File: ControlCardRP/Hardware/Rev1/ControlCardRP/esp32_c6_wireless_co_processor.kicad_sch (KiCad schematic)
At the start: 22 parts, among them J6 ESP_PROG_UART, J7 ESP_PROG_JTAG, J8 ESP_IO, SW103 NRST, SW104 NRST, U5 ESP32-C6-MINI-1

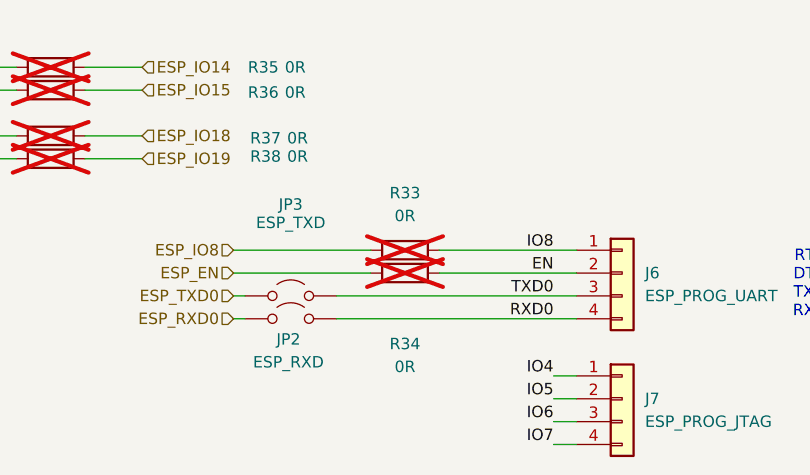
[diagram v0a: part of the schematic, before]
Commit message: A
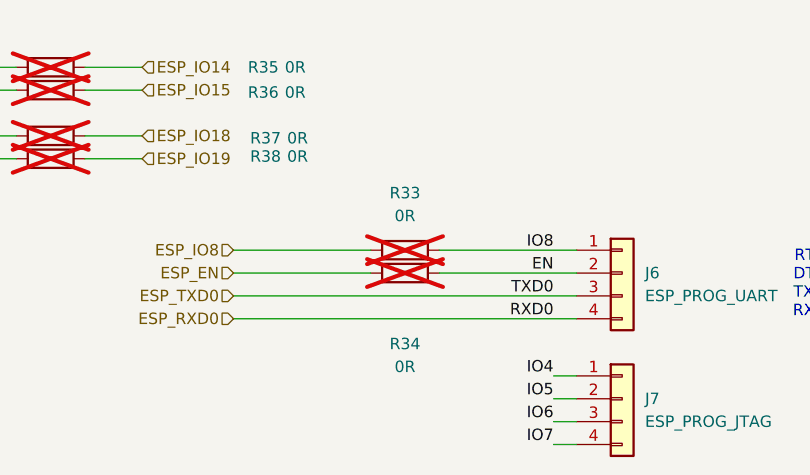
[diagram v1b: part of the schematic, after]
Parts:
- removed JP2: ESP_RXD, Connector_PinHeader_1.27mm:PinHeader_1x02_P1.27mm_Vertical, symbol Jumper:Jumper_2_Open
- removed JP3: ESP_TXD, Connector_PinHeader_1.27mm:PinHeader_1x02_P1.27mm_Vertical, symbol Jumper:Jumper_2_Open
- J6, J7: footprint (none) -> Connector_PinHeader_1.27mm:PinHeader_1x04_P1.27mm_Vertical
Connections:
- net RXD0 is gone; now on net ESP_RXD0: J6.4 (Pin_4), U5.30 (RXD0)
- net TXD0 is gone; now on net ESP_TXD0: J6.3 (Pin_3), U5.31 (TXD0)
